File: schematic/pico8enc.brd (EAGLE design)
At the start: 200.6 x 34 mm, 10 parts, among them U1 RASPBERRY_PICOSMD-TH

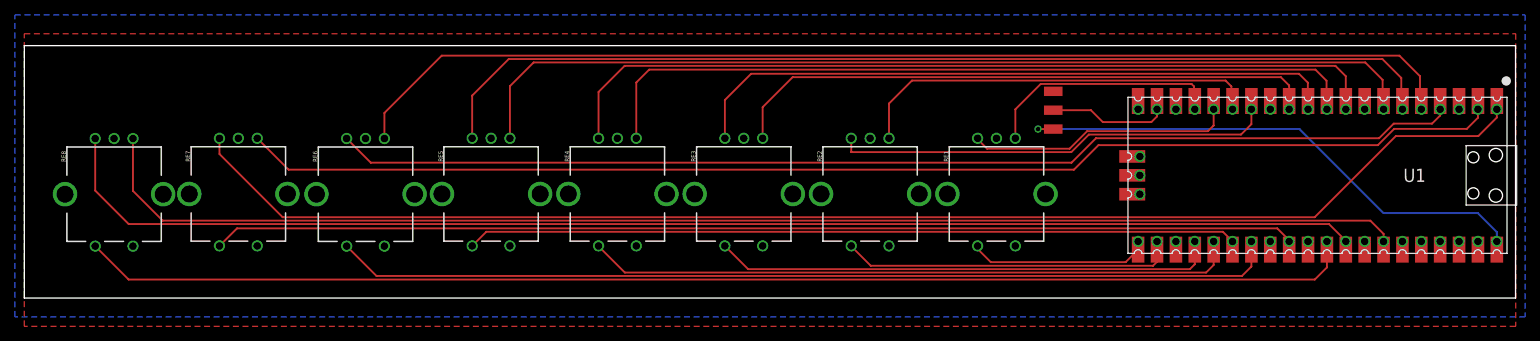
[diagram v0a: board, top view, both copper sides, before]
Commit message: pcb cleanup
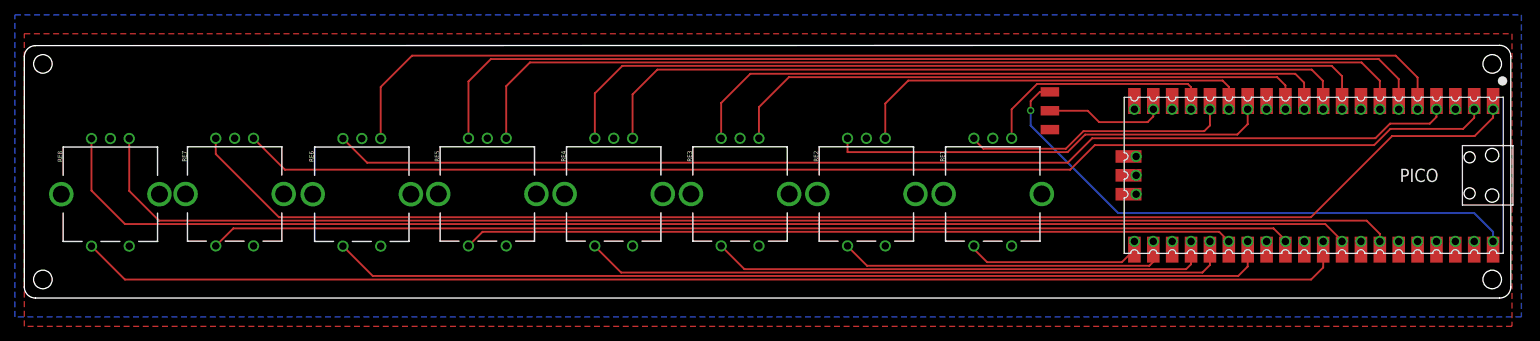
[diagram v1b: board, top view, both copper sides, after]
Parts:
- removed U1: RASPBERRY_PICOSMD-TH, RpiPico:PICO-PKG
- added PICO: RASPBERRY_PICOSMD-TH, RpiPico:PICO-PKG
- moved RE1 0.50 mm to (130.3, 14.0)
- moved RE2 0.50 mm to (113.3, 14.0)
- moved RE3 0.50 mm to (96.3, 14.0)
- moved RE4 0.50 mm to (79.3, 14.0)
- moved RE5 0.50 mm to (62.3, 14.0)
- moved RE6 0.50 mm to (45.4, 14.0)
- moved RE7 0.50 mm to (28.3, 14.0)
- moved RE8 0.50 mm to (11.6, 14.0)
- moved JP1 0.44 mm to (138.0, 25.2), turned to 270 degrees
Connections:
- net 3V3(OUT): now also PICO.36, PICO.P$36; no longer U1.36, U1.P$36
- net GND: now also PICO.13, PICO.18, PICO.23, PICO.28, PICO.3, PICO.33, PICO.38, PICO.8, PICO.P$13, PICO.P$18, PICO.P$23, PICO.P$28, PICO.P$3, PICO.P$33, PICO.P$38, PICO.P$8; no longer U1.13, U1.18, U1.23, U1.28, U1.3, U1.33, U1.38, U1.8, U1.P$13, U1.P$18, U1.P$23, U1.P$28, U1.P$3, U1.P$33, U1.P$38, U1.P$8
- net N$1: now also PICO.17, PICO.P$17; no longer U1.17, U1.P$17
- net N$10: now also PICO.6, PICO.P$6; no longer U1.6, U1.P$6
- net N$11: now also PICO.5, PICO.P$5; no longer U1.5, U1.P$5
- net N$12: now also PICO.4, PICO.P$4; no longer U1.4, U1.P$4
- net N$13: now also PICO.2, PICO.P$2; no longer U1.2, U1.P$2
- net N$14: now also PICO.1, PICO.P$1; no longer U1.1, U1.P$1
- net N$15: now also PICO.34, PICO.P$34; no longer U1.34, U1.P$34
- net N$16: now also PICO.32, PICO.P$32; no longer U1.32, U1.P$32
- net N$2: now also PICO.16, PICO.P$16; no longer U1.16, U1.P$16
- net N$3: now also PICO.15, PICO.P$15; no longer U1.15, U1.P$15
- net N$4: now also PICO.14, PICO.P$14; no longer U1.14, U1.P$14
- net N$5: now also PICO.12, PICO.P$12; no longer U1.12, U1.P$12
- net N$6: now also PICO.11, PICO.P$11; no longer U1.11, U1.P$11
- net N$7: now also PICO.10, PICO.P$10; no longer U1.10, U1.P$10
- net N$8: now also PICO.9, PICO.P$9; no longer U1.9, U1.P$9
- net N$9: now also PICO.7, PICO.P$7; no longer U1.7, U1.P$7
- net RE1SW: now also PICO.21, PICO.P$21; no longer U1.21, U1.P$21
- net RE2SW: now also PICO.22, PICO.P$22; no longer U1.22, U1.P$22
- net RE3SW: now also PICO.24, PICO.P$24; no longer U1.24, U1.P$24
- net RE4SW: now also PICO.25, PICO.P$25; no longer U1.25, U1.P$25
- net RE5SW: now also PICO.26, PICO.P$26; no longer U1.26, U1.P$26
- net RE6SW: now also PICO.27, PICO.P$27; no longer U1.27, U1.P$27
- net RE7SW: now also PICO.29, PICO.P$29; no longer U1.29, U1.P$29
- net RE8SW: now also PICO.31, PICO.P$31; no longer U1.31, U1.P$31
- net SECRETNEOPIXELS: now also PICO.19, PICO.P$19; no longer U1.19, U1.P$19
- net SWGND: now also PICO.42, PICO.P$42; no longer U1.42, U1.P$42
- net VBUS: now also PICO.40, PICO.P$40; no longer U1.40, U1.P$40
- net VSYS: now also PICO.39, PICO.P$39; no longer U1.39, U1.P$39
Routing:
- net VBUS: track 71.9 -> 76.9 mm
- net N$1: track 34.9 -> 32.6 mm
- net N$7: track 107.0 -> 104.6 mm
- net N$9: track 133.0 -> 130.7 mm
- net N$6: track 90.5 -> 88.9 mm
- net N$3: track 56.9 -> 55.5 mm
- net N$11: track 153.0 -> 153.7 mm
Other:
- board size 200.6 x 34 mm -> 200 x 34 mm
